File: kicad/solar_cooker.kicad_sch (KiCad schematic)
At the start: 7 parts, among them U1 ATmega2560-16A, U2 microSD, U3 clock_module, U4 e-Paper, U5 anemometer

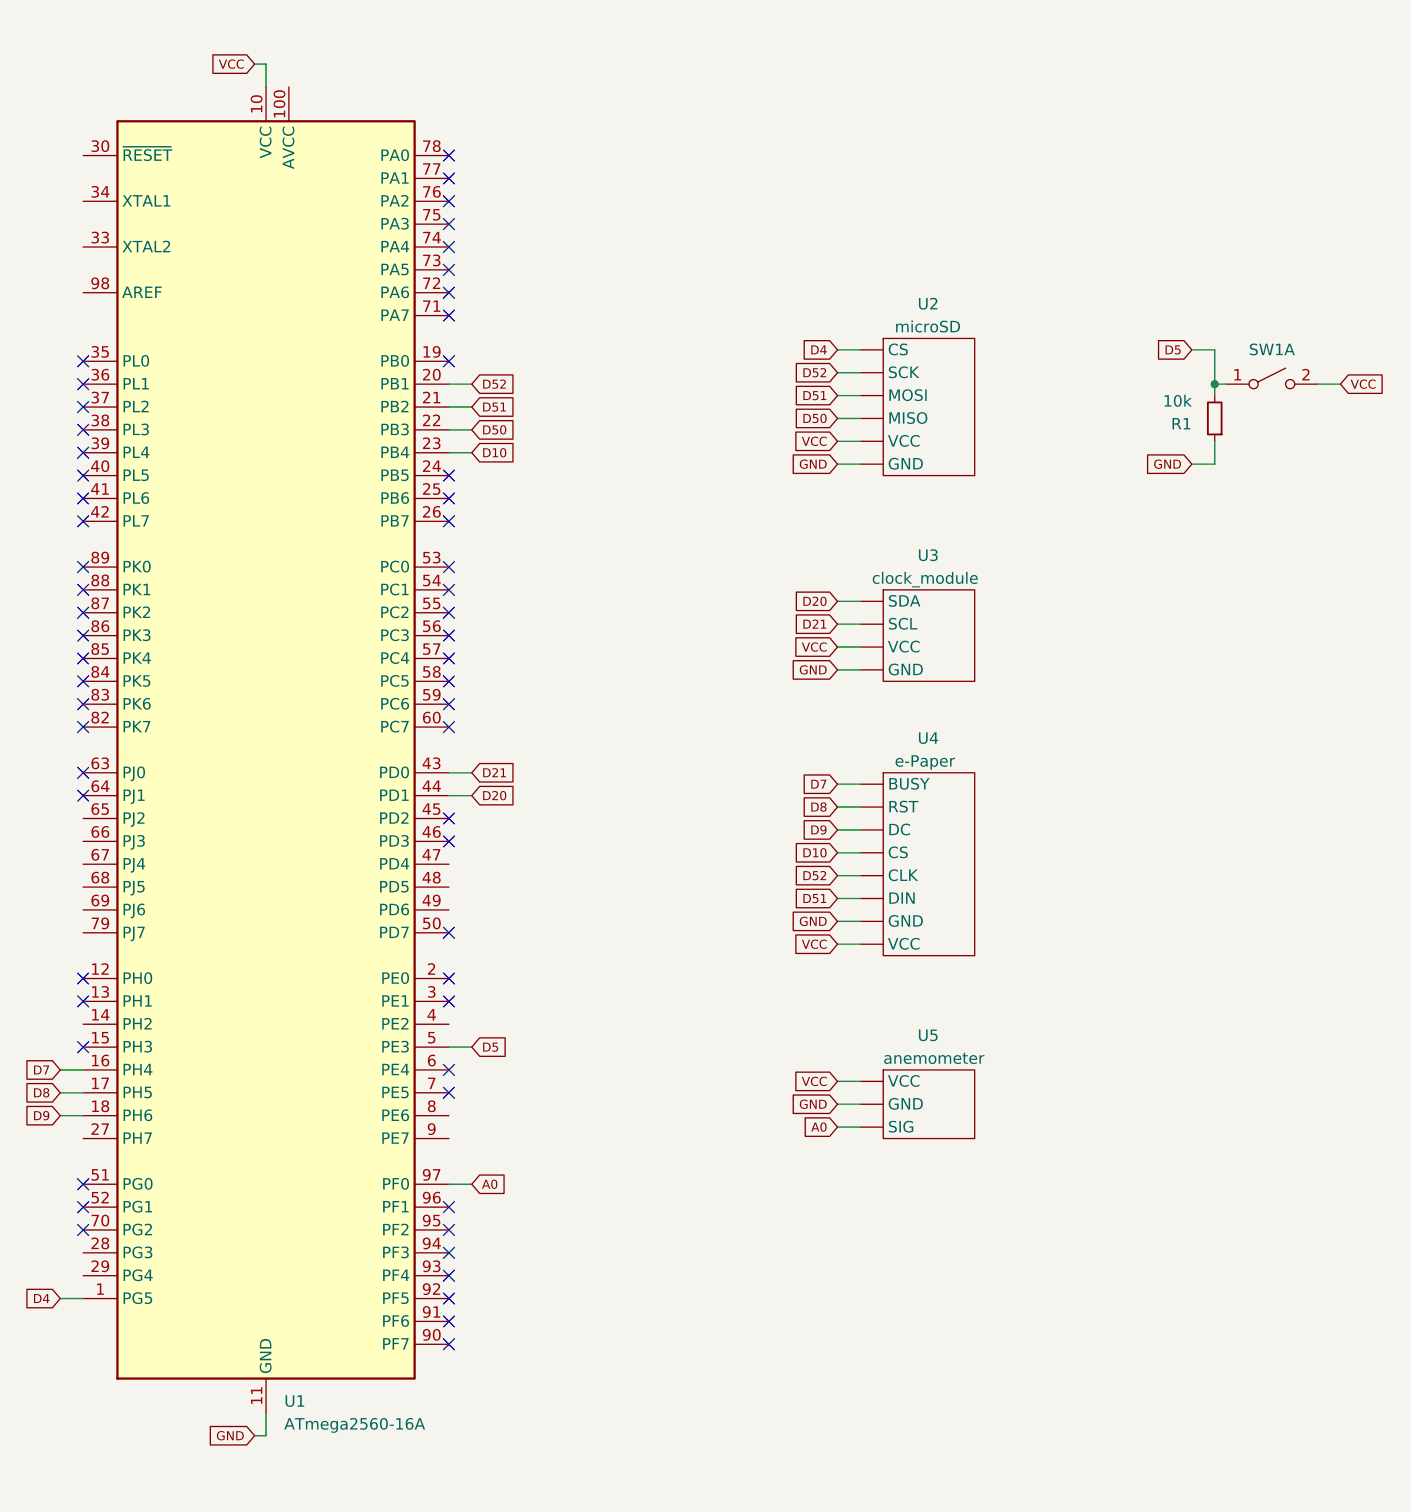
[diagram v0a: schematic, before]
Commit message: schematic and documentation update
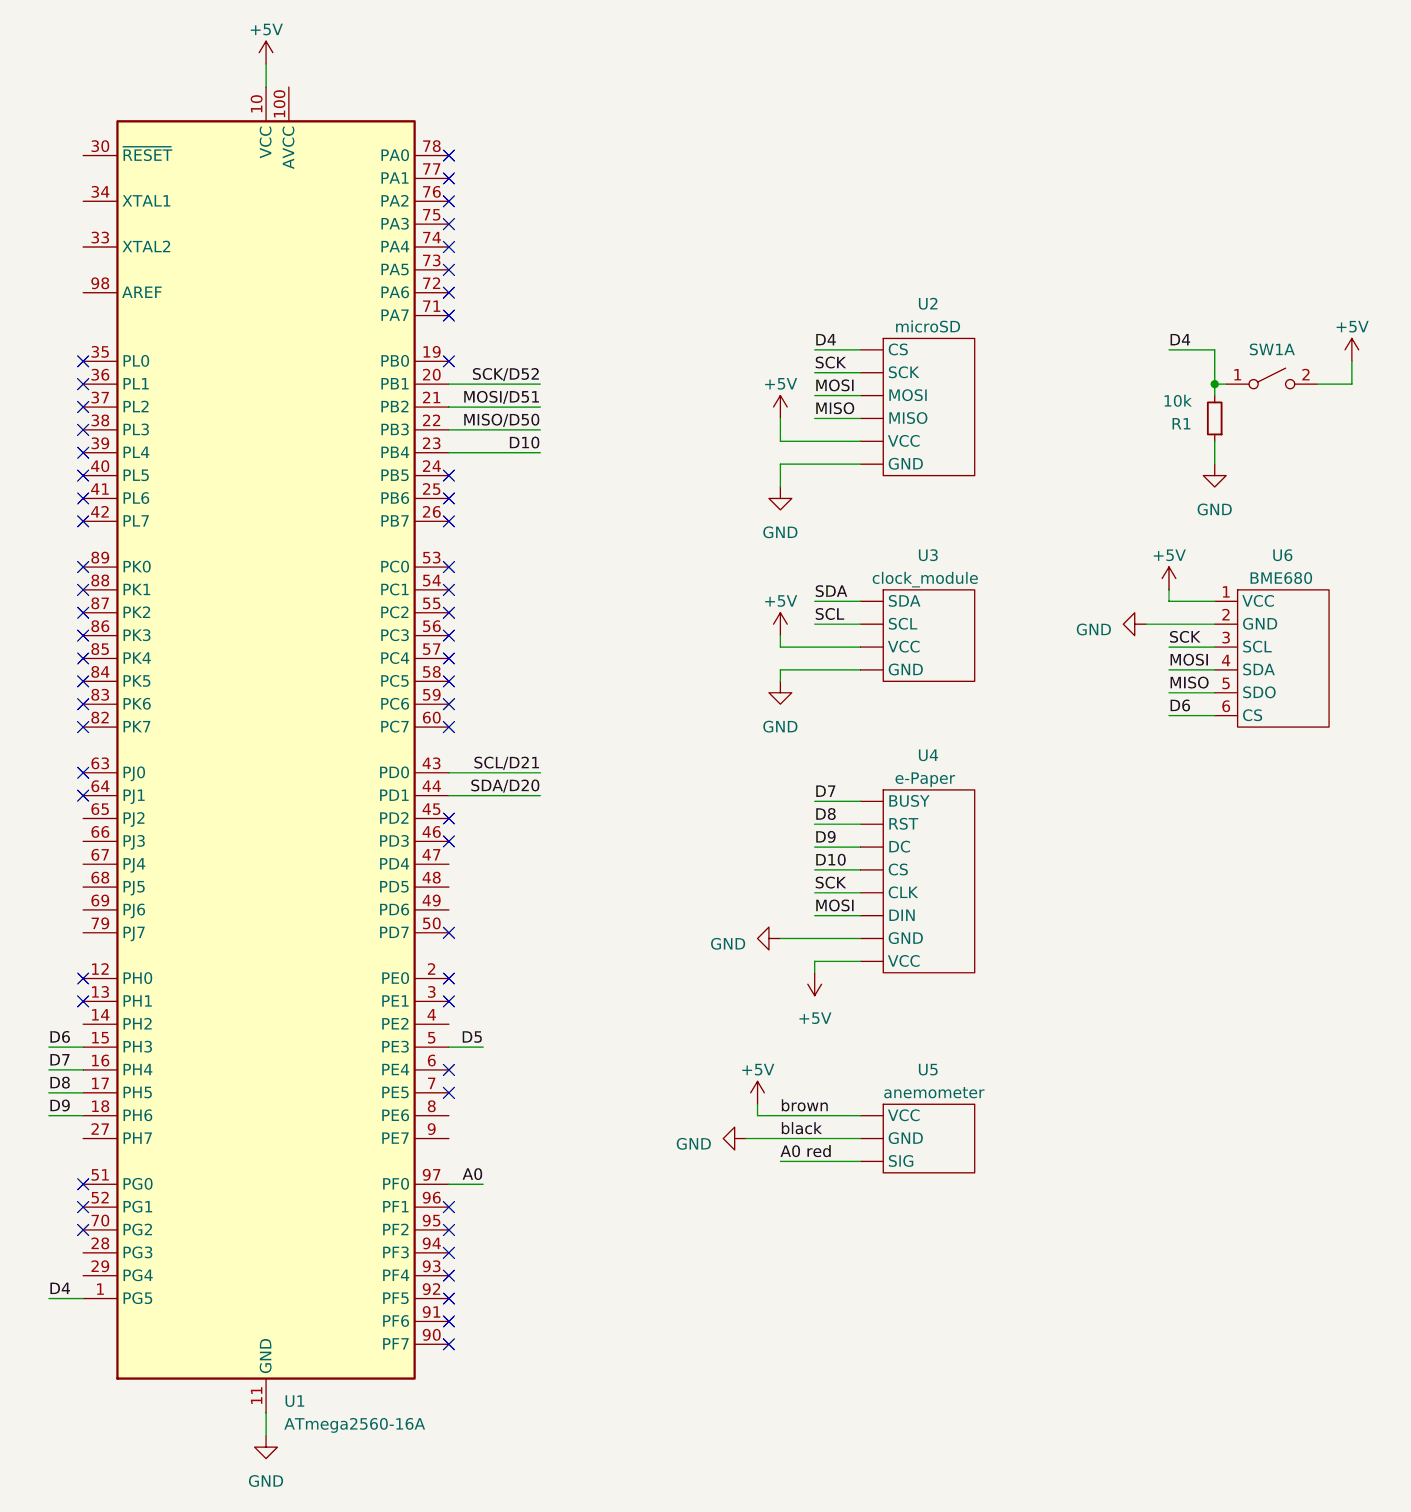
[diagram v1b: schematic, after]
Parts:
- added U6: BME680, symbol custom_components:BME680
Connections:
- net A0: no longer U5.3 (SIG)
- net D4: now also R1.2, SW1.1 (A)
- net D5: no longer R1.2, SW1.1 (A)
- net GND: now also U6.2 (GND)
- net D6: now reaches U1.15 (PH3)
- net D6: now also U6.6 (CS)
- net D20 renamed SDA
- net SDA: no longer U1.44 (PD1)
- net D21 renamed SCL
- net SCL: no longer U1.43 (PD0)
- net D50 renamed MISO
- net MISO: now also U6.5 (SDO); no longer U1.22 (PB3)
- net D51 renamed MOSI
- net MOSI: now also U6.4 (SDA); no longer U1.21 (PB2)
- net D52 renamed SCK
- net SCK: now also U6.3 (SCL); no longer U1.20 (PB1)
- net VCC renamed +5V
- net +5V: now also U6.1 (VCC)
- new net A0 red: U5.3 (SIG)
- new net MISO/D50: U1.22 (PB3)
- new net MOSI/D51: U1.21 (PB2)
- new net SCK/D52: U1.20 (PB1)
- new net SCL/D21: U1.43 (PD0)
- new net SDA/D20: U1.44 (PD1)
- no-connect marks 58 -> 57
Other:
- moved on the sheet: U4, U5
